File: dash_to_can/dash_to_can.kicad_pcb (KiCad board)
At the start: 2 copper layers, 100 x 100 mm, 64 parts, among them J1 AVR-ISP1, J2 Conn_02x10_Top_Bottom, Q1 2N3904, Q10 AO3401A, Q2 2N3904, Q3 2N3904, Q4 AO3401A, Q5 2N3904, Q6 AO3401A, Q7 2N3904, Q8 AO3401A, Q9 2N3904, U1 ATmega328P-A, U2 LM2575-5.0BU, U3 MCP2515-xST, U4 TJA1050T_CM_118, U5 ULN2003A, U6 MCP41010, Y1 20MHz, Y2 16MHz

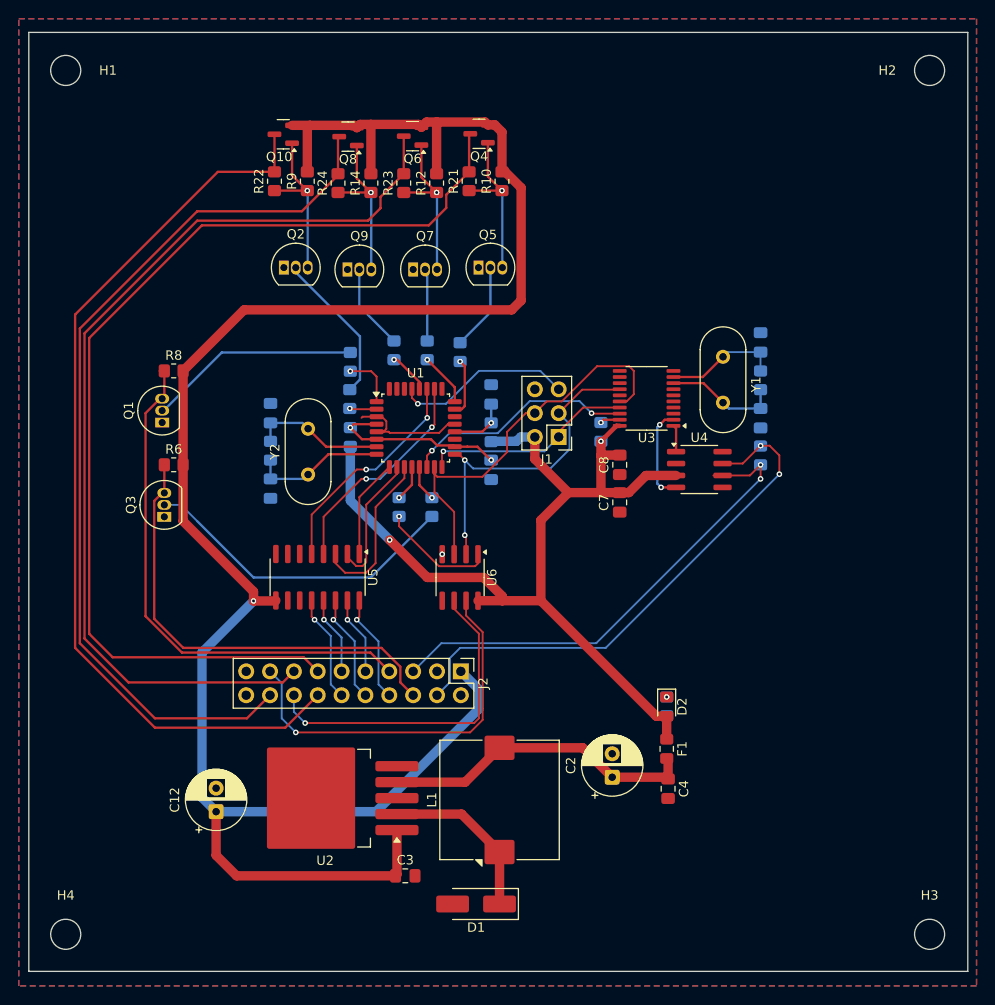
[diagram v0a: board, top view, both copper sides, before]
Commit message: Second Draft
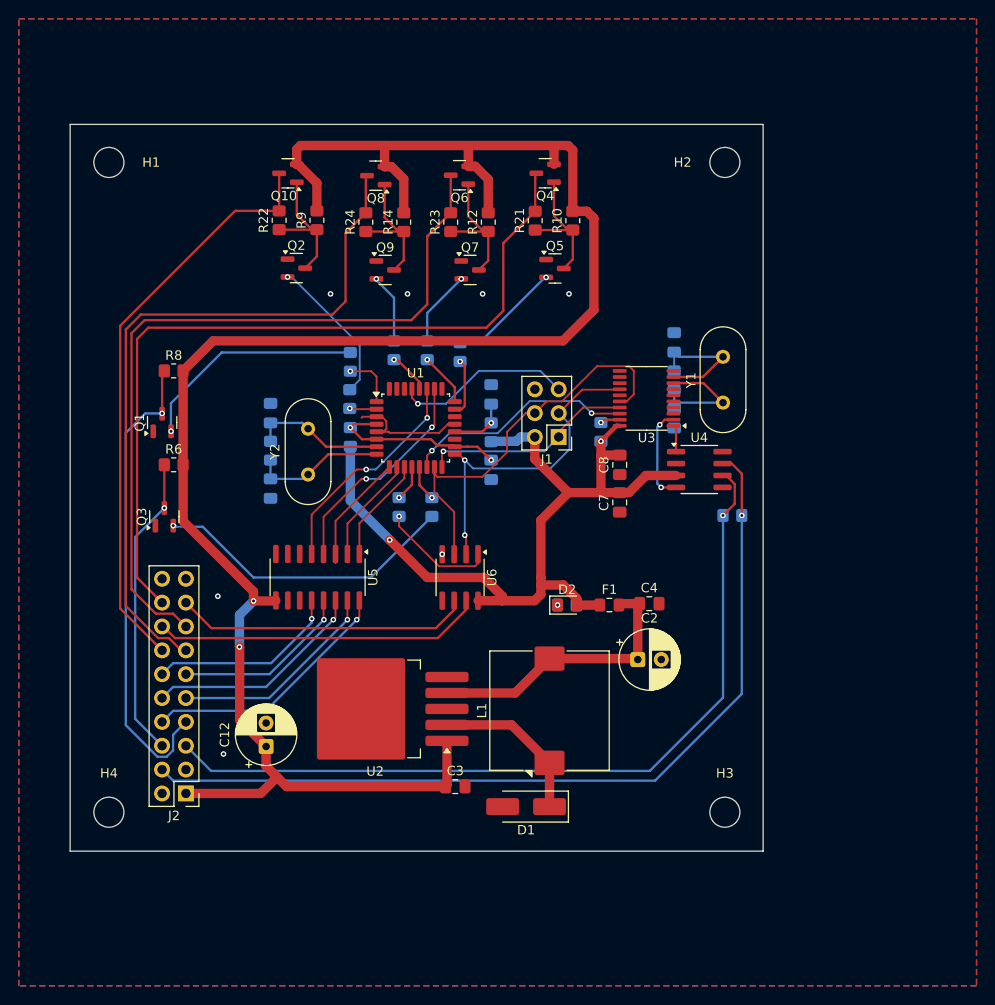
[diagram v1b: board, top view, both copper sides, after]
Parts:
- Q1, Q2, Q3, Q5, Q7, Q9: footprint Package_TO_SOT_THT:TO-92_Inline -> Package_TO_SOT_SMD:SOT-23
- moved J2 32.0 mm to (90.8, 109.0), turned to 180 degrees
- moved H3 25.4 mm to (148.2, 111.0)
- moved H2 23.9 mm to (148.2, 41.8)
- moved C4 19.8 mm to (140.2, 88.8), turned to 0 degrees
- moved F1 16.5 mm to (135.9, 88.9), turned to 0 degrees
- moved R17 15.1 mm to (131.4, 88.9), turned to 180 degrees
- moved D2 15.1 mm to (131.4, 88.9), turned to 0 degrees
- moved H4 13.8 mm to (82.6, 111.0)
- moved C2 12.8 mm to (138.9, 94.7), turned to 0 degrees
- moved D1 11.7 mm to (127.0, 110.4)
- moved C3 10.9 mm to (119.5, 108.3)
- moved L1 10.9 mm to (129.5, 100.2)
- moved U2 10.9 mm to (111.0, 100.0)
- moved H1 10.8 mm to (82.6, 41.8)
- moved C5 9.20 mm to (142.8, 69.0)
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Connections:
- J2 pad 16: FUEL -> TEMP
- J2 pad 17: TEMP -> FUEL
- Q4 pad 3: TURN R -> ILLUM
- Q5 pad 2: R DRIVER -> ILLUM DRIVER
- Q8 pad 3: ILLUM -> TURN R
- Q9 pad 2: ILLUM DRIVER -> R DRIVER
- R11 pad 2: R DRIVER -> ILLUM DRIVER
- R13 pad 2: ILLUM DRIVER -> R DRIVER
- R21 pad 2: TURN R -> ILLUM
- R24 pad 2: ILLUM -> TURN R
- U1 pad 11: D3 -> D1
- U1 pad 9: D1 -> D3
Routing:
- net TURN L: track 97.8 -> 62.4 mm
- net CANL: track 52.5 -> 87.7 mm, vias 2 -> 1
- net CANH: track 57.0 -> 92.0 mm, vias 2 -> 1
- net TURN R: track 110.2 -> 76.8 mm
- net HI BEAM: track 103.0 -> 82.3 mm
- net TACHO: track 48.9 -> 32.4 mm, vias 0 -> 1
- net Neutral: track 11.6 -> 27.4 mm
- net Oil: track 8.35 -> 22.7 mm
- net +5V: track 102.2 -> 88.4 mm
- net +12V: track 219.6 -> 206.4 mm, vias 1 -> 2
- net FI IND: track 11.6 -> 23.8 mm
- net ILLUM: track 96.5 -> 85.5 mm
- net HESD IND: track 8.35 -> 19.2 mm
- net IMMOBI IND: track 11.4 -> 20.6 mm
- net TEMP: track 41.5 -> 35.1 mm, vias 1 -> 0
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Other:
- board size 100 x 100 mm -> 73.8 x 77.4 mm
